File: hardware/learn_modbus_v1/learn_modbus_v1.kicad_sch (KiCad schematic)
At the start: 11 parts, among them J1 SJ-43514-SMT, J3 RTU_CONN, U2 SeeeduinoXIAO, U3 THD301D485H

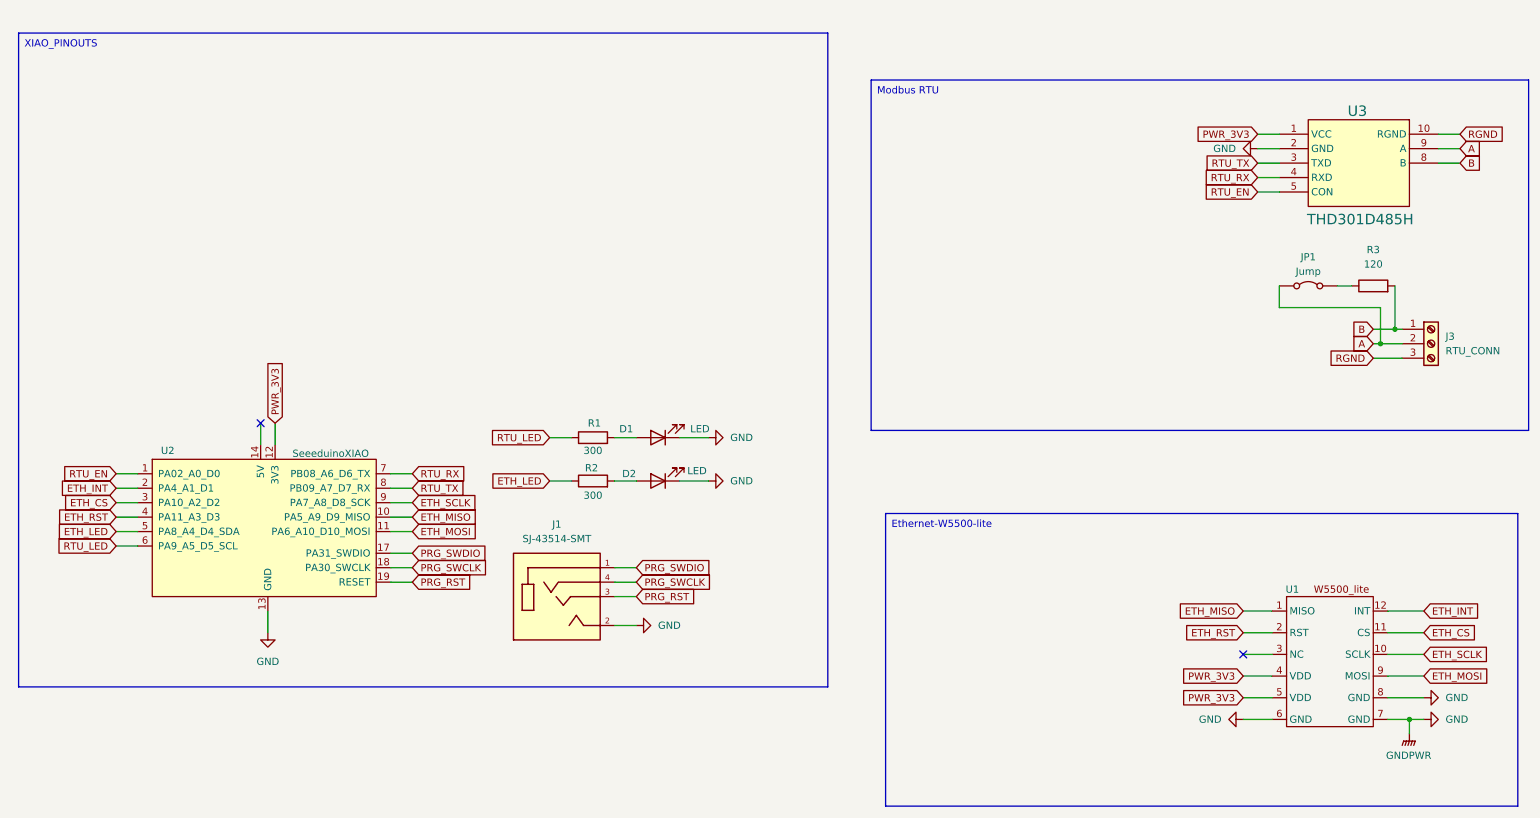
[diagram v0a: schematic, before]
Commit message: hardware init
hardware init
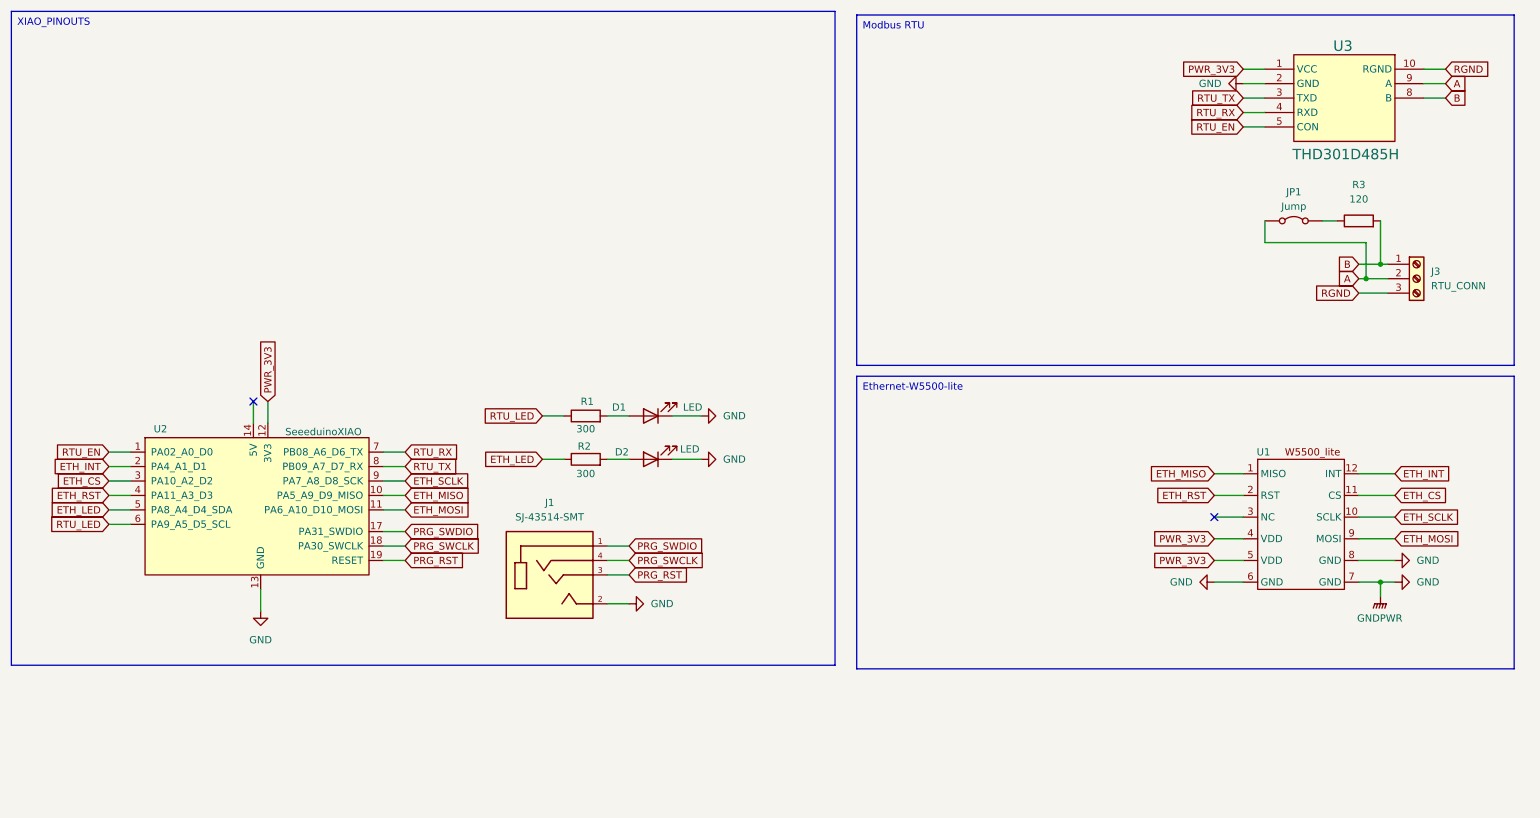
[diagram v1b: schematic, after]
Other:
- moved on the sheet: D1, D2, J1, J3, JP1, R1, R2, R3, U1, U2, U3
